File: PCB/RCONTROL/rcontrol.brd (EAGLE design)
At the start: 26.6 x 45.4 mm, 13 parts

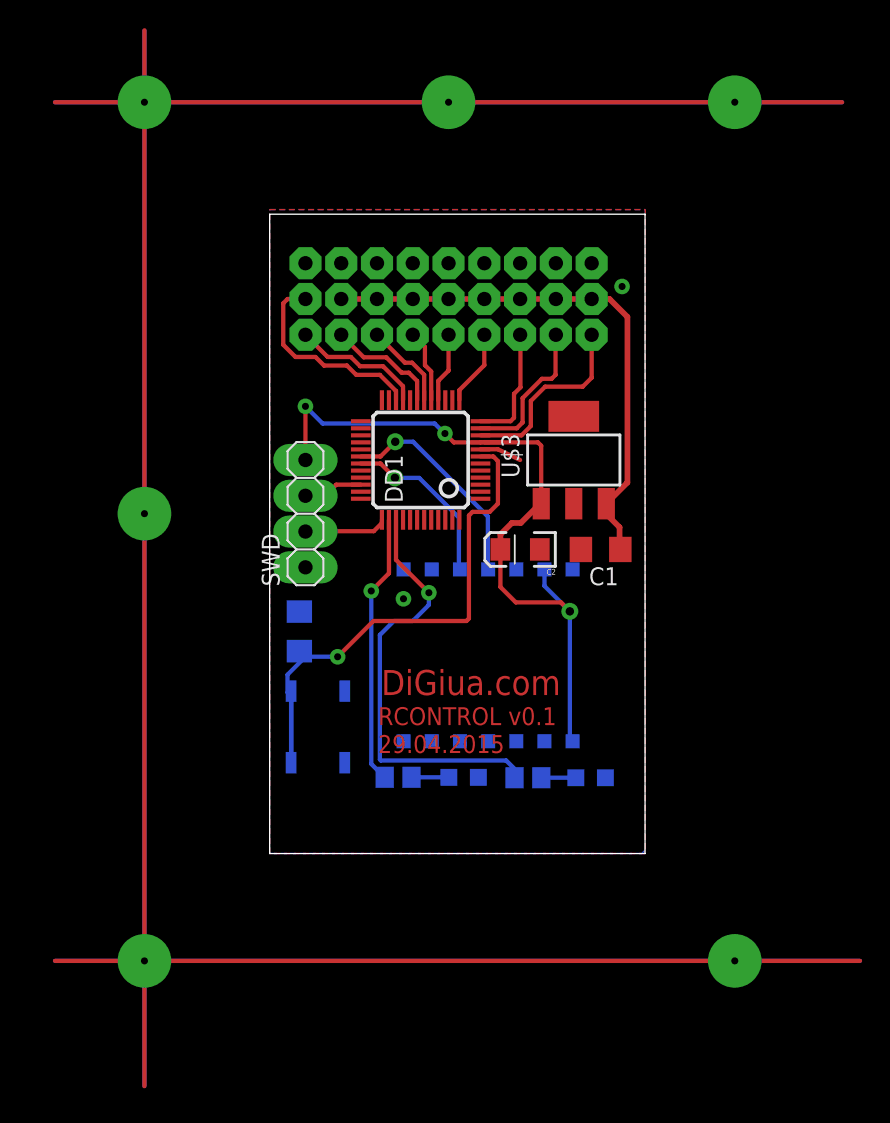
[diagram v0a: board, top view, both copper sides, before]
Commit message: New PCB
New PCB
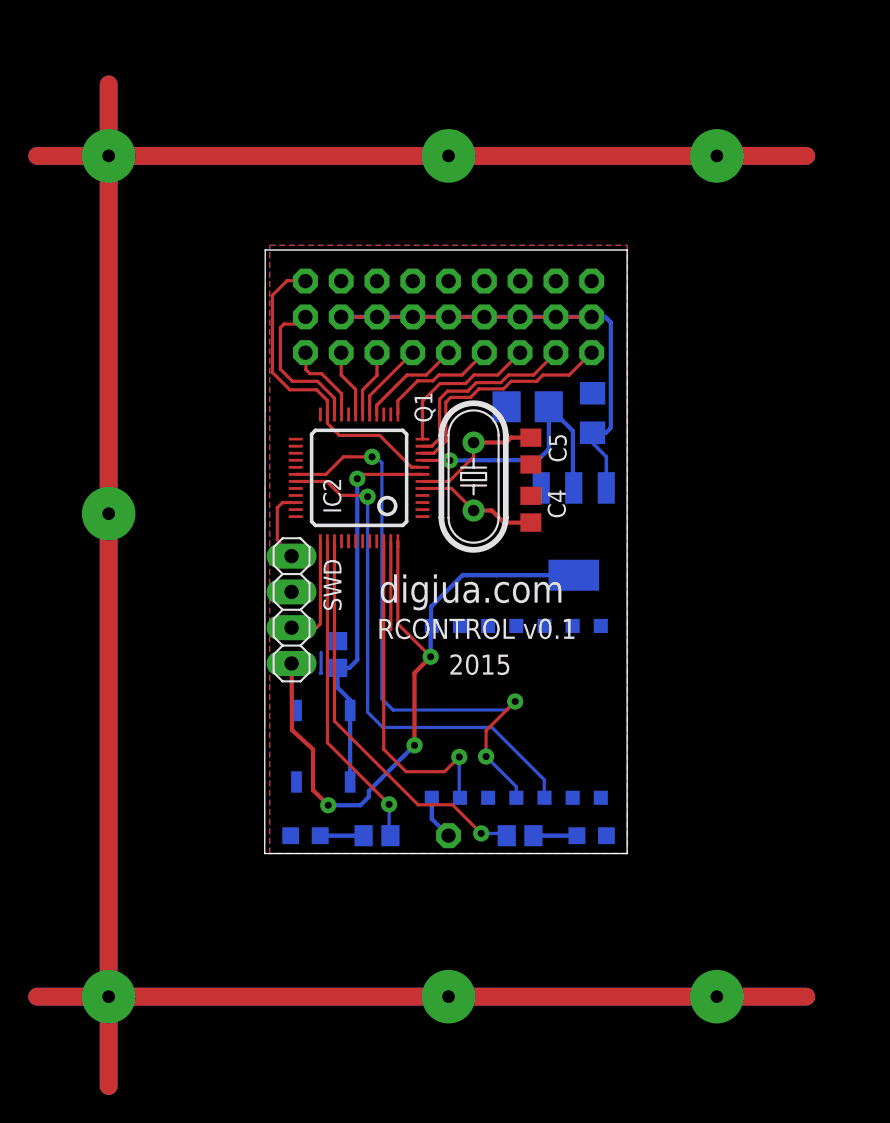
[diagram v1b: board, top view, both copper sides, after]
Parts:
- removed DD1: (no value), pepelac:LQFP48
- removed LED1, LED2: (no value), led:CHIP-LED0805
- removed U$1: ESP8266_ESP-03, ESP8266:ESP-03
- removed U$2: (no value), pinhead:3X09
- removed U$3: LD333.3, lm1117:SOT223
- added ANT: (no value), pinhead:1X01
- added C4, C5: 22pF, rcl:C0805
- added ESP8266: ESP8266_ESP-03, ESP8266:ESP-03
- added GREEN, RED: (no value), led:CHIP-LED0805
- added IC1: LM1117IMPX-3.3, lm1117:SOT223
- added IC2: STM32F10XCXT6, STM32:TQFP48
- added Q1: 8MHz, crystal:HC49U-V
- added U1: PINHD3X9, pinheader3x9:3X9
- C2: value 1uF -> 1uf; device SparkFun-Capacitors:EIA3216 -> rcl:CT3528
- C3: device rcl:C1206 -> rcl:C0805
- moved C2 10.1 mm to (18.3, 31.7), flipped to the bottom, turned to 0 degrees
- moved C1 9.70 mm to (22.9, 31.3), flipped to the bottom, turned to 90 degrees
- moved SWD 6.90 mm to (1.56, 17.3), turned to 270 degrees
- moved R1 4.40 mm to (7.62, 1.27), turned to 180 degrees
- moved R2 4.15 mm to (17.8, 1.27)
- moved C3 3.12 mm to (4.76, 14.1)
- moved S1 1.42 mm to (3.81, 7.62), turned to 270 degrees
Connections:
- new net N$19: ESP8266.6, IC2.46
- new net N$36: C3.1, IC2.7, S1.3, S1.4
- new net N$37: C5.1, IC2.6, Q1.2
- new net N$9: ANT.1, ESP8266.7
- new net VBAT: IC2.1
- net +3V3: now also C2.+, ESP8266.8, IC1.2, IC1.TAB, IC2.24, IC2.36, IC2.48, IC2.9; no longer C2.A, DD1.9, U$1.6, U$1.8, U$3.1
- net GND: now also C2.-, C4.2, C5.2, ESP8266.1, ESP8266.12, GREEN.C, IC1.1, IC2.23, IC2.35, IC2.47, IC2.8, RED.C, SWD.2, U1.12, U1.15, U1.18, U1.21, U1.24, U1.27, U1.3, U1.6, U1.9; no longer C2.C, DD1.8, LED1.C, LED2.C, SWD.1, U$1.1, U$1.12, U$2.021, U$2.12, U$2.15, U$2.18, U$2.24, U$2.27, U$2.3, U$2.6, U$2.9, U$3.2, U$3.TAB
- net N$1: now also IC2.10, U1.1; no longer DD1.30, U$1.4
- net N$10: now also IC2.19, U1.22; no longer DD1.10, U$2.1
- net N$11: now also IC2.21, U1.25; no longer DD1.11, U$2.4
- net N$12: now also IC2.22, U1.26; no longer DD1.12, U$2.7
- net N$13: now also ESP8266.4, IC2.30; no longer DD1.13, U$2.10
- net N$14: now also ESP8266.3, IC2.31; no longer DD1.16, U$2.13
- net N$15: now also IC2.34, SWD.1; no longer DD1.17, U$2.16
- net N$16: now also IC2.37, SWD.3; no longer DD1.18, U$2.19
- net N$17: now also IC2.38, R1.2; no longer DD1.19, U$2.022
- net N$18: now also IC2.39, R2.2; no longer DD1.22, U$2.26
- net N$2: now also IC2.11, U1.4; no longer DD1.31, U$1.3
- net N$20: now also RED.A; no longer LED1.A
- net N$21: now also GREEN.A; no longer LED2.A
- net N$23: now also IC1.3, U1.11, U1.14, U1.17, U1.2, U1.20, U1.23, U1.5, U1.8; no longer U$2.020, U$2.023, U$2.11, U$2.14, U$2.17, U$2.2, U$2.5, U$2.8, U$3.3
- net N$3: now also IC2.12, U1.7; no longer DD1.34, SWD.3
- net N$4: now also IC2.13, U1.10; no longer DD1.21, U$2.25
- net N$5: now also IC2.16, U1.13; no longer DD1.37, SWD.2
- net N$6: now also C4.1, IC2.5, Q1.1; no longer C3.1, DD1.7, S1.3, S1.4
- net N$7: now also IC2.17, U1.16; no longer DD1.38, R1.2
- net N$8: now also IC2.18, U1.19; no longer DD1.39, R2.2
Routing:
- net N$28: track 75.0 -> 0.00 mm, vias 0 -> 1
- net N$34: track 0.00 -> 71.1 mm
- net N$30: track 55.9 -> 0.00 mm, vias 0 -> 1
- net N$35: track 0.00 -> 54.6 mm
- net N$13: track 5.37 -> 42.2 mm, vias 0 -> 3
- net N$6: track 40.7 -> 8.70 mm, vias 1 -> 0
- net N$14: track 4.94 -> 36.7 mm, vias 0 -> 1
- net N$36: track 0.00 -> 27.8 mm, vias 0 -> 1
- net GND: track 2.99 -> 30.2 mm, vias 2 -> 0
- net N$8: track 30.7 -> 4.81 mm, vias 1 -> 0
- net N$19: track 1.27 -> 24.1 mm, vias 0 -> 1
- net N$29: track 74.9 -> 54.6 mm
- net +3V3: track 52.0 -> 68.7 mm, vias 3 -> 4
- net N$31: track 55.9 -> 71.1 mm
- net N$17: track 8.11 -> 22.8 mm, vias 0 -> 1
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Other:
- board size 26.6 x 45.4 mm -> 25.7 x 42.9 mm
- board text added: "2015"
- board text added: "digiua.com"
- board text removed: "29.04.2015"
- board text removed: "DiGiua.com"
